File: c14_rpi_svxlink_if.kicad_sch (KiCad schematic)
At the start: 54 parts, among them J1 RPi_GPIO Tall, J2 Conn_01x04, J3 Conn_01x04, J4 Conn_01x04, J5 Conn_01x02, J6 Conn_01x04, J7 DB9F, Q1 BC847, Q2 BC847, Q3 BC847, Q4 BC857, Q5 BC847, T1 1:1, T2 1:1, U1 TLP222A o. AQY282EH, U2 HCPL-B17, U3 ADS1115_Module

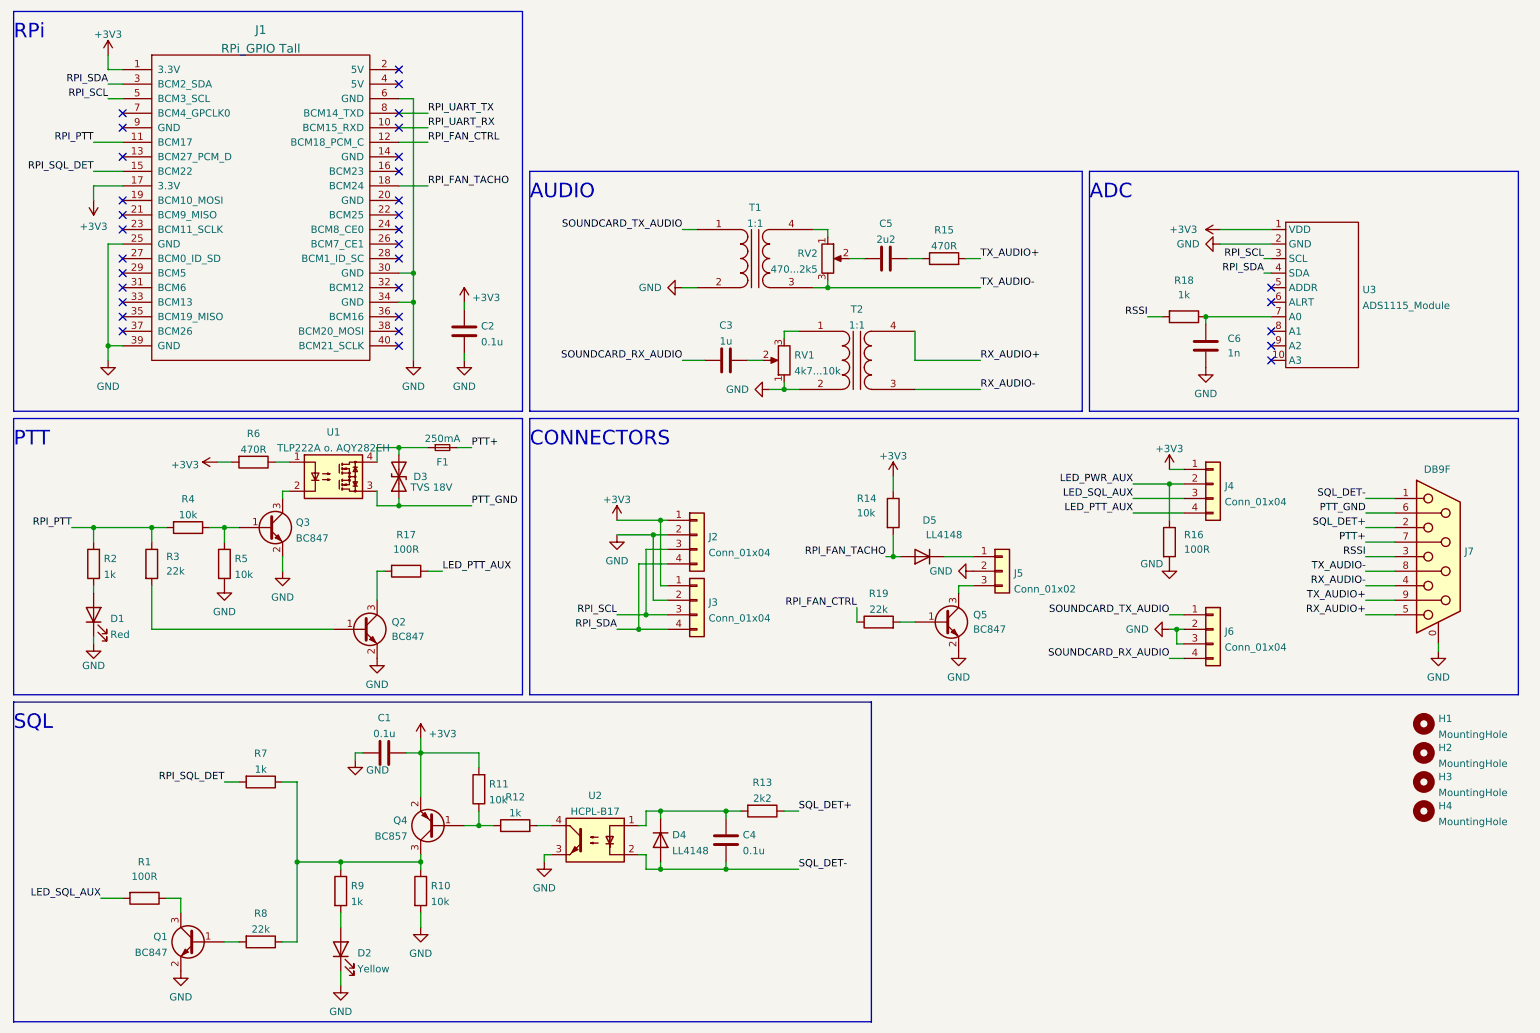
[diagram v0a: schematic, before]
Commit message: Neue Teile platziert, pre-1.1 bereit fuer Review
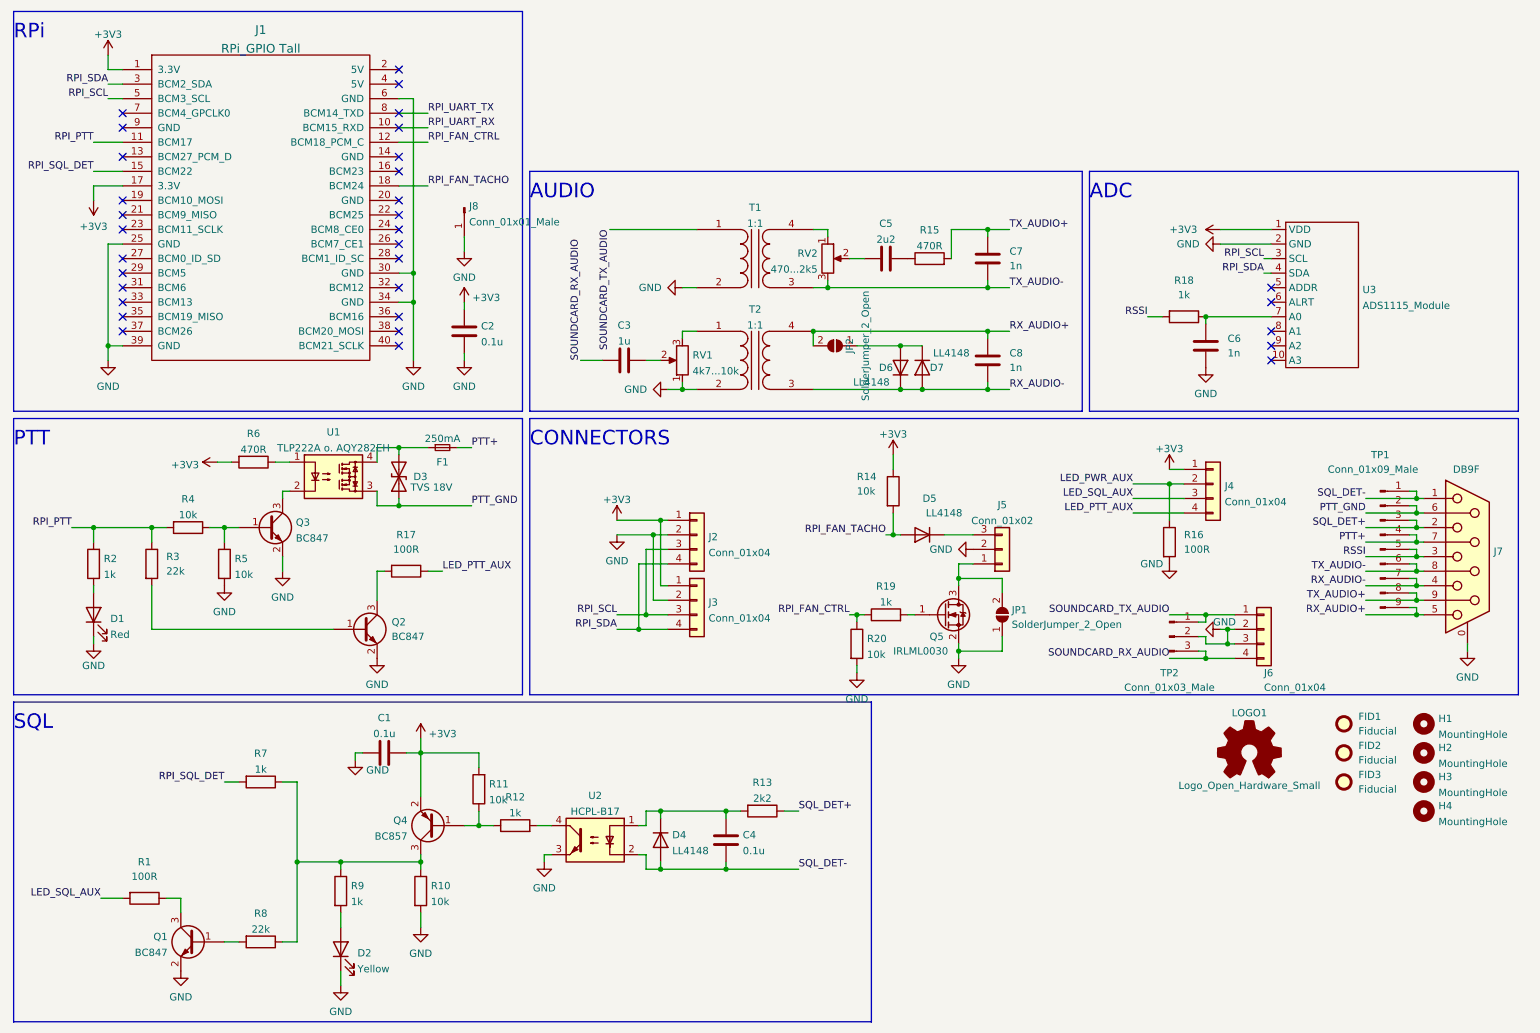
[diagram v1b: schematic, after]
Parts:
- removed Q5: BC847, Package_TO_SOT_SMD:SOT-23, symbol Transistor_BJT:BC847
- added C7, C8: 1n, Capacitor_SMD:C_0805_2012Metric_Pad1.18x1.45mm_HandSolder, symbol Device:C
- added D6, D7: LL4148, Diode_SMD:D_MiniMELF, symbol Diode:LL4148
- added FID1, FID2, FID3: Fiducial, Fiducial:Fiducial_1mm_Mask3mm, symbol Mechanical:Fiducial
- added J8: Conn_01x01_Male, Connector_PinHeader_2.54mm:PinHeader_1x01_P2.54mm_Vertical, symbol Connector:Conn_01x01_Male
- added JP1, JP2: SolderJumper_2_Open, Jumper:SolderJumper-2_P1.3mm_Open_TrianglePad1.0x1.5mm, symbol Jumper:SolderJumper_2_Open
- added LOGO1: Logo_Open_Hardware_Small, Symbol:OSHW-Logo2_9.8x8mm_SilkScreen, symbol Graphic:Logo_Open_Hardware_Small
- added Q5: IRLML0030, Package_TO_SOT_SMD:SOT-23, symbol Transistor_FET:IRLML0030
- added R20: 10k, Resistor_SMD:R_0805_2012Metric_Pad1.20x1.40mm_HandSolder, symbol Device:R
- added TP1: Conn_01x09_Male, Connector_PinHeader_1.27mm:PinHeader_1x09_P1.27mm_Vertical, symbol Connector:Conn_01x09_Male
- added TP2: Conn_01x03_Male, Connector_PinHeader_1.27mm:PinHeader_1x03_P1.27mm_Vertical, symbol Connector:Conn_01x03_Male
- R19: value 22k -> 1k
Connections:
- net GND: now also J8.1 (Pin_1), JP1.1 (A), Q5.2 (S), R20.2, TP2.2 (Pin_2)
- net PTT+: now also TP1.4 (Pin_4)
- net PTT_GND: now also TP1.2 (Pin_2)
- net RPI_FAN_CTRL: now also R20.1
- net RSSI: now also TP1.5 (Pin_5)
- net RX_AUDIO+: now also C8.2, JP2.2 (B), TP1.9 (Pin_9)
- net RX_AUDIO-: now also C8.1, D6.1 (K), D7.2 (A), TP1.7 (Pin_7)
- net SOUNDCARD_RX_AUDIO: now also TP2.3 (Pin_3)
- net SOUNDCARD_TX_AUDIO: now also TP2.1 (Pin_1)
- net SQL_DET+: now also TP1.3 (Pin_3)
- net SQL_DET-: now also TP1.1 (Pin_1)
- net TX_AUDIO+: now also C7.2, TP1.8 (Pin_8)
- net TX_AUDIO-: now also C7.1, TP1.6 (Pin_6)
- net at R19.2: now also Q5.1 (G)
- net at J5.1 (Pin_1): now also JP1.2 (B), Q5.3 (D); no longer D5.1 (K)
- net at J5.3 (Pin_3): now also D5.1 (K)
- new net: D6.2 (A), D7.1 (K), JP2.1 (A)
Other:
- moved on the sheet: C3, D5, J5, J6, J7, R14, R15, R19, RV1, T2
